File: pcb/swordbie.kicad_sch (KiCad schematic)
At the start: 10 parts, among them J1 Conn_01x08_Pin, J2 Conn_01x04_Pin, SW1 SW_Push, SW2 SW_Push, U1 XIAO-ESP32-C3-SMD, U2 DHT11

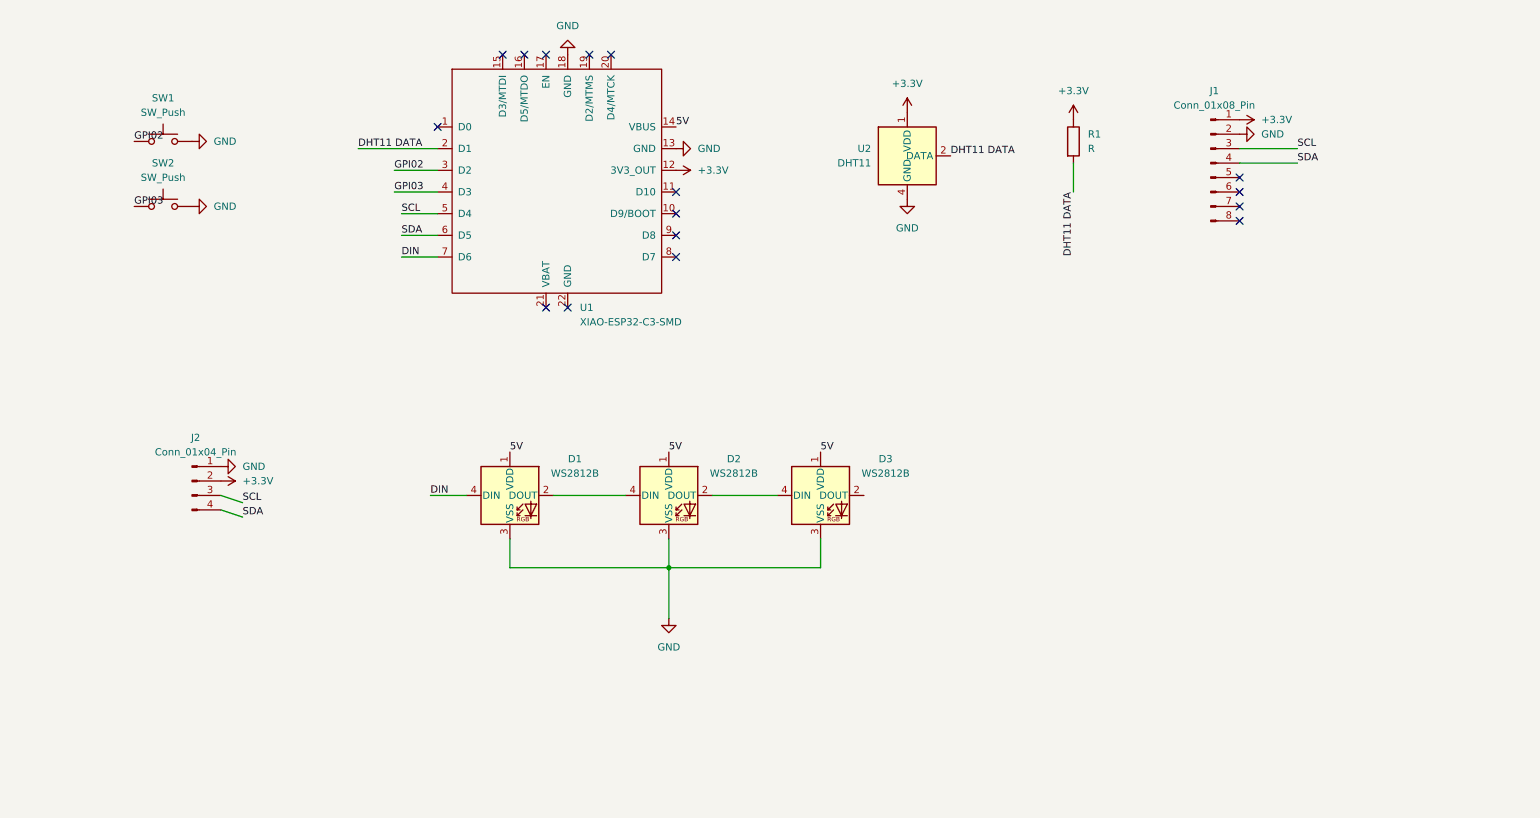
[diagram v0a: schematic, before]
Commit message: new pcb files updated design
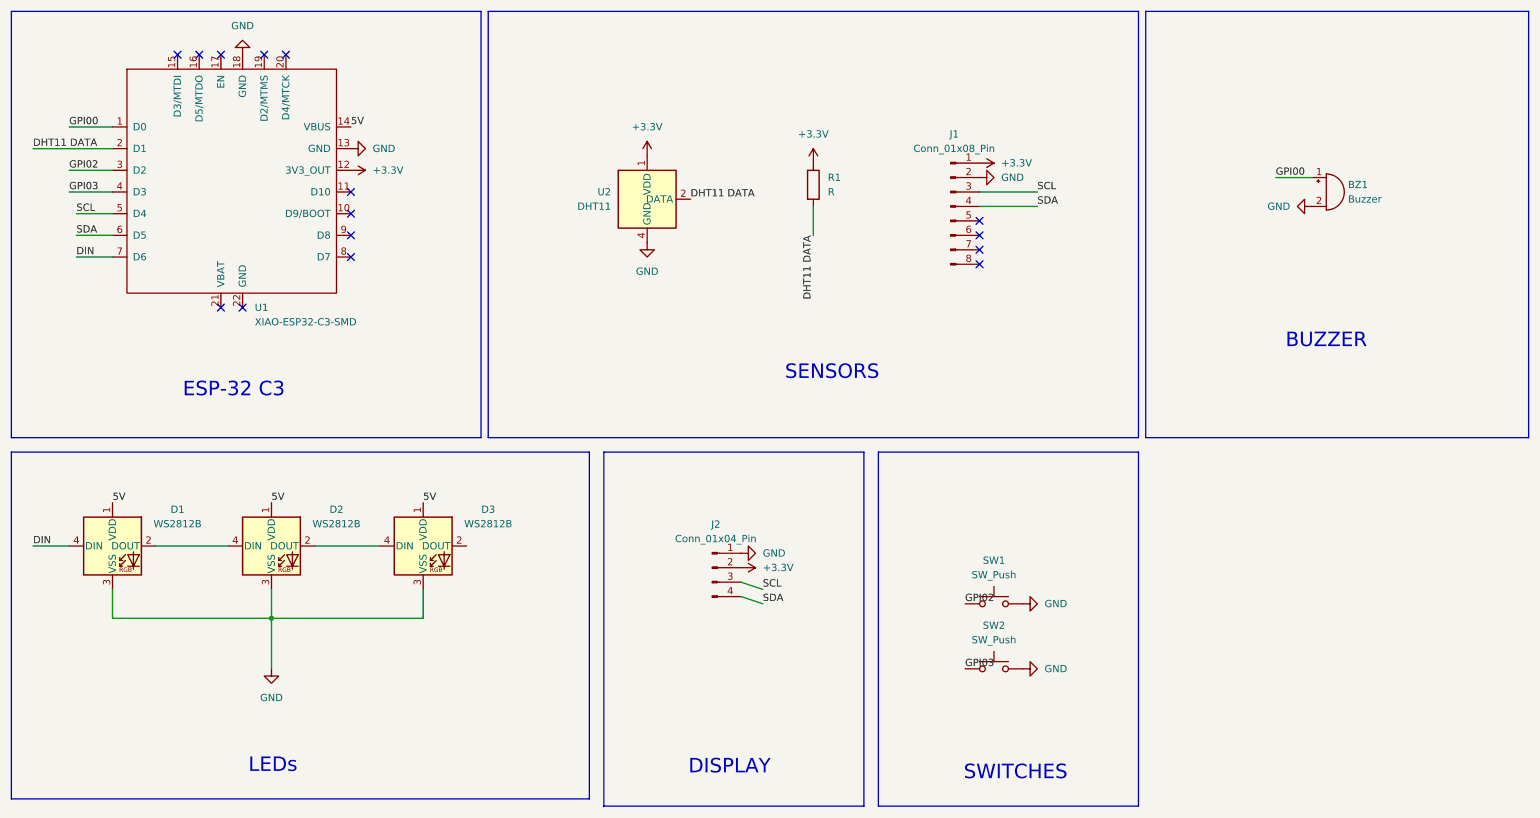
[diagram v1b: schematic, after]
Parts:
- added BZ1: Buzzer, Buzzer_Beeper:Buzzer_12x9.5RM7.6, symbol Device:Buzzer
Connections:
- net GND: now also BZ1.2 (-)
- net GPI00: now reaches U1.1 (D0)
- net GPI00: now also BZ1.1 (+)
- no-connect marks 16 -> 15
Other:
- note added: "BUZZER"
- note added: "DISPLAY"
- note added: "ESP-32 C3"
- note added: "LEDs"
- note added: "SENSORS"
- note added: "SWITCHES"
- moved on the sheet: D1, D2, D3, J1, J2, R1, SW1, SW2, U1, U2
